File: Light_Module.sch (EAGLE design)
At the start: 67 parts, among them IC1 TLC59711, IC2 TLC59711

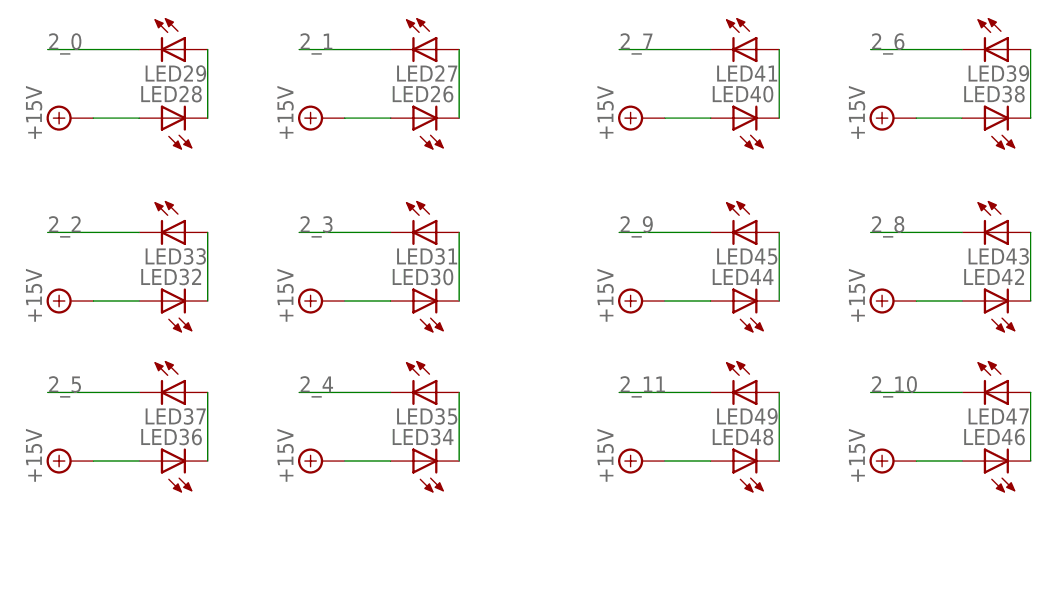
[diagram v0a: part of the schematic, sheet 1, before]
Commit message: delete some
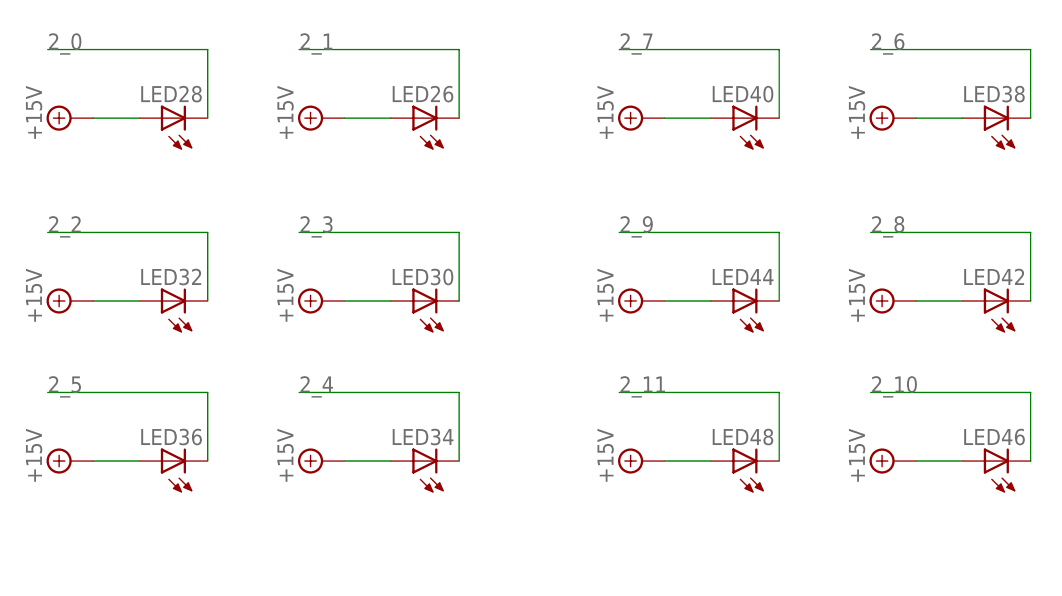
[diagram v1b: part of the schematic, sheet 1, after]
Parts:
- removed LED27, LED29, LED31, LED33, LED35, LED37, LED39, LED41, LED43, LED45, LED47, LED49: (no value), digikey:LED
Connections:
- removed net N$20: LED26.C, LED27.A
- removed net N$21: LED28.C, LED29.A
- removed net N$22: LED30.C, LED31.A
- removed net N$23: LED32.C, LED33.A
- removed net N$24: LED34.C, LED35.A
- removed net N$25: LED36.C, LED37.A
- removed net N$26: LED38.C, LED39.A
- removed net N$27: LED40.C, LED41.A
- removed net N$28: LED42.C, LED43.A
- removed net N$29: LED44.C, LED45.A
- removed net N$30: LED46.C, LED47.A
- removed net N$31: LED48.C, LED49.A
- net 2_0: now also LED28.C; no longer LED29.C
- net 2_1: now also LED26.C; no longer LED27.C
- net 2_10: now also LED46.C; no longer LED47.C
- net 2_11: now also LED48.C; no longer LED49.C
- net 2_2: now also LED32.C; no longer LED33.C
- net 2_3: now also LED30.C; no longer LED31.C
- net 2_4: now also LED34.C; no longer LED35.C
- net 2_5: now also LED36.C; no longer LED37.C
- net 2_6: now also LED38.C; no longer LED39.C
- net 2_7: now also LED40.C; no longer LED41.C
- net 2_8: now also LED42.C; no longer LED43.C
- net 2_9: now also LED44.C; no longer LED45.C

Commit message: Revert 42a1a8e..717766d
This rolls back to commit 42a1a8ecaa921d949cbaf7c99d83dff5afafc410.
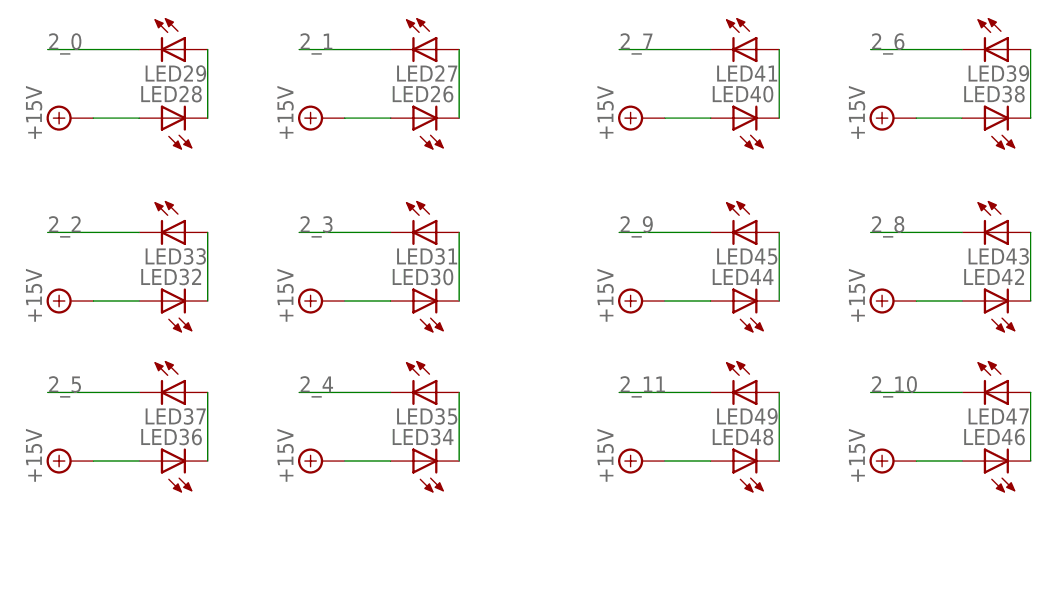
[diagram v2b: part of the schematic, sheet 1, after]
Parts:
- added LED27, LED29, LED31, LED33, LED35, LED37, LED39, LED41, LED43, LED45, LED47, LED49: (no value), digikey:LED
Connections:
- new net N$20: LED26.C, LED27.A
- new net N$21: LED28.C, LED29.A
- new net N$22: LED30.C, LED31.A
- new net N$23: LED32.C, LED33.A
- new net N$24: LED34.C, LED35.A
- new net N$25: LED36.C, LED37.A
- new net N$26: LED38.C, LED39.A
- new net N$27: LED40.C, LED41.A
- new net N$28: LED42.C, LED43.A
- new net N$29: LED44.C, LED45.A
- new net N$30: LED46.C, LED47.A
- new net N$31: LED48.C, LED49.A
- net 2_0: now also LED29.C; no longer LED28.C
- net 2_1: now also LED27.C; no longer LED26.C
- net 2_10: now also LED47.C; no longer LED46.C
- net 2_11: now also LED49.C; no longer LED48.C
- net 2_2: now also LED33.C; no longer LED32.C
- net 2_3: now also LED31.C; no longer LED30.C
- net 2_4: now also LED35.C; no longer LED34.C
- net 2_5: now also LED37.C; no longer LED36.C
- net 2_6: now also LED39.C; no longer LED38.C
- net 2_7: now also LED41.C; no longer LED40.C
- net 2_8: now also LED43.C; no longer LED42.C
- net 2_9: now also LED45.C; no longer LED44.C
